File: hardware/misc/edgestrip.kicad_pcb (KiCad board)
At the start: 2 copper layers, 6 x 24.1 mm, 2 parts

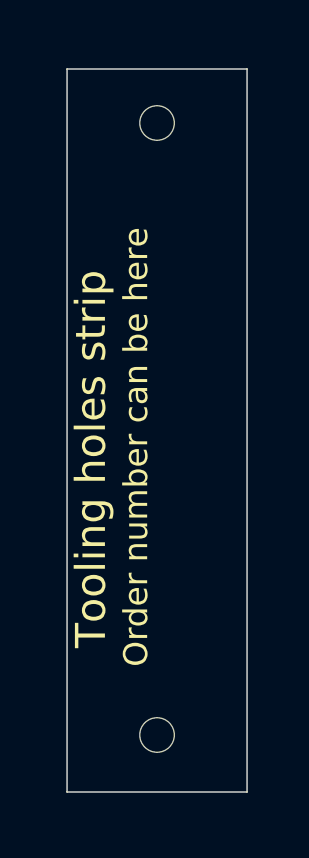
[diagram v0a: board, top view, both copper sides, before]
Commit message: Panelisation stuff
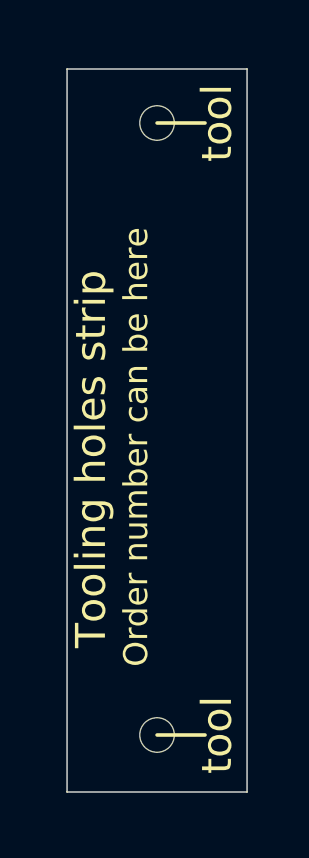
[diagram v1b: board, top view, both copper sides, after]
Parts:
- turned REF** to 90 degrees (x2)
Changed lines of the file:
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@@
-(kicad_pcb (version 20200119) (host pcbnew "5.99.0-unknown-9de7547~100~ubuntu18.04.1")
+(kicad_pcb (version 20200119) (host pcbnew "5.99.0-unknown-4f36980~101~ubuntu18.04.1")
   (general
     (thickness 1.6)
@@
       (usegerberadvancedattributes false)
       (creategerberjobfile false)
+      (svguseinch false)
+      (svgprecision 6)
       (excludeedgelayer true)
       (linewidth 0.100000)
@@
   )
   (module "misc:toolhole" (layer "F.Cu")
-    (at 133 82.2)
-    (fp_text reference "REF**" (at 0 2.54 unlocked) (layer "F.SilkS") hide
+    (at 133 82.2 90)
+    (fp_text reference "REF**" (at 0 2.54 90 unlocked) (layer "F.SilkS") hide
       (effects (font (size 1 1) (thickness 0.15)))
     )
-    (fp_text value "toolhole" (at 0 -2.54 unlocked) (layer "F.Fab")
+    (fp_text value "toolhole" (at 0 -2.54 90 unlocked) (layer "F.Fab")
       (effects (font (size 1 1) (thickness 0.15)))
     )
-    (pad "" np_thru_hole circle (at 0 0) (size 1.152 1.152) (drill 1.152) (layers *.Cu *.Mask)
-      (solder_mask_margin 0.148))
+    (fp_text user "tool" (at 0 2 90 unlocked) (layer "F.SilkS")
+      (effects (font (size 1 1) (thickness 0.15)))
+    )
+    (fp_line (start 0 1.6) (end 0 0) (layer "F.SilkS") (width 0.12))
+    (pad "" np_thru_hole circle (at 0 0 90) (size 1.152 1.152) (drill 1.152) (layers *.Cu *.Mask)
+      (solder_mask_margin 0.6))
   )
   (module "misc:toolhole" (layer "F.Cu")
-    (at 133 61.8)
-    (fp_text reference "REF**" (at 0 2.54 unlocked) (layer "F.SilkS") hide
+    (at 133 61.8 90)
+    (fp_text reference "REF**" (at 0 2.54 90 unlocked) (layer "F.SilkS") hide
       (effects (font (size 1 1) (thickness 0.15)))
     )
-    (fp_text value "toolhole" (at 0 -2.54 unlocked) (layer "F.Fab")
+    (fp_text value "toolhole" (at 0 -2.54 90 unlocked) (layer "F.Fab")
       (effects (font (size 1 1) (thickness 0.15)))
     )
-    (pad "" np_thru_hole circle (at 0 0) (size 1.152 1.152) (drill 1.152) (layers *.Cu *.Mask)
-      (solder_mask_margin 0.148))
+    (fp_text user "tool" (at 0 2 90 unlocked) (layer "F.SilkS")
+      (effects (font (size 1 1) (thickness 0.15)))
+    )
+    (fp_line (start 0 1.6) (end 0 0) (layer "F.SilkS") (width 0.12))
+    (pad "" np_thru_hole circle (at 0 0 90) (size 1.152 1.152) (drill 1.152) (layers *.Cu *.Mask)
+      (solder_mask_margin 0.6))
   )
   (gr_text "Order number can be here" (at 132.3 72.6 90) (layer "F.SilkS")
